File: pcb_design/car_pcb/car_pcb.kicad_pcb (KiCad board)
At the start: 2 copper layers, 158 x 115 mm, 28 parts, among them J1 PICO_R, J10 CMD_UART, J11 +5V, J12 PICO_L, J14 PWR_OUTPUT, J16 NRF24L01, J18 GND, J19 +3.3V, J2 PWR_INPUT, J20 GND, J21 PWR_IN_BTN, J22 Joystick_Y_PWR_GND, J23 Joystick_Y_SIGs, J24 Camera servo, J3 Joystick_X_PWR_GND, J4 Joystick_X_SIGs, J5 Motor_1, J6 Motor_2, J7 Motor_3, J8 Motor_4, J9 Debug_UART, U2 Mini360_5V, U3 Mini360_3.3V, U4 module_mpu6050, U5 ROB-14450

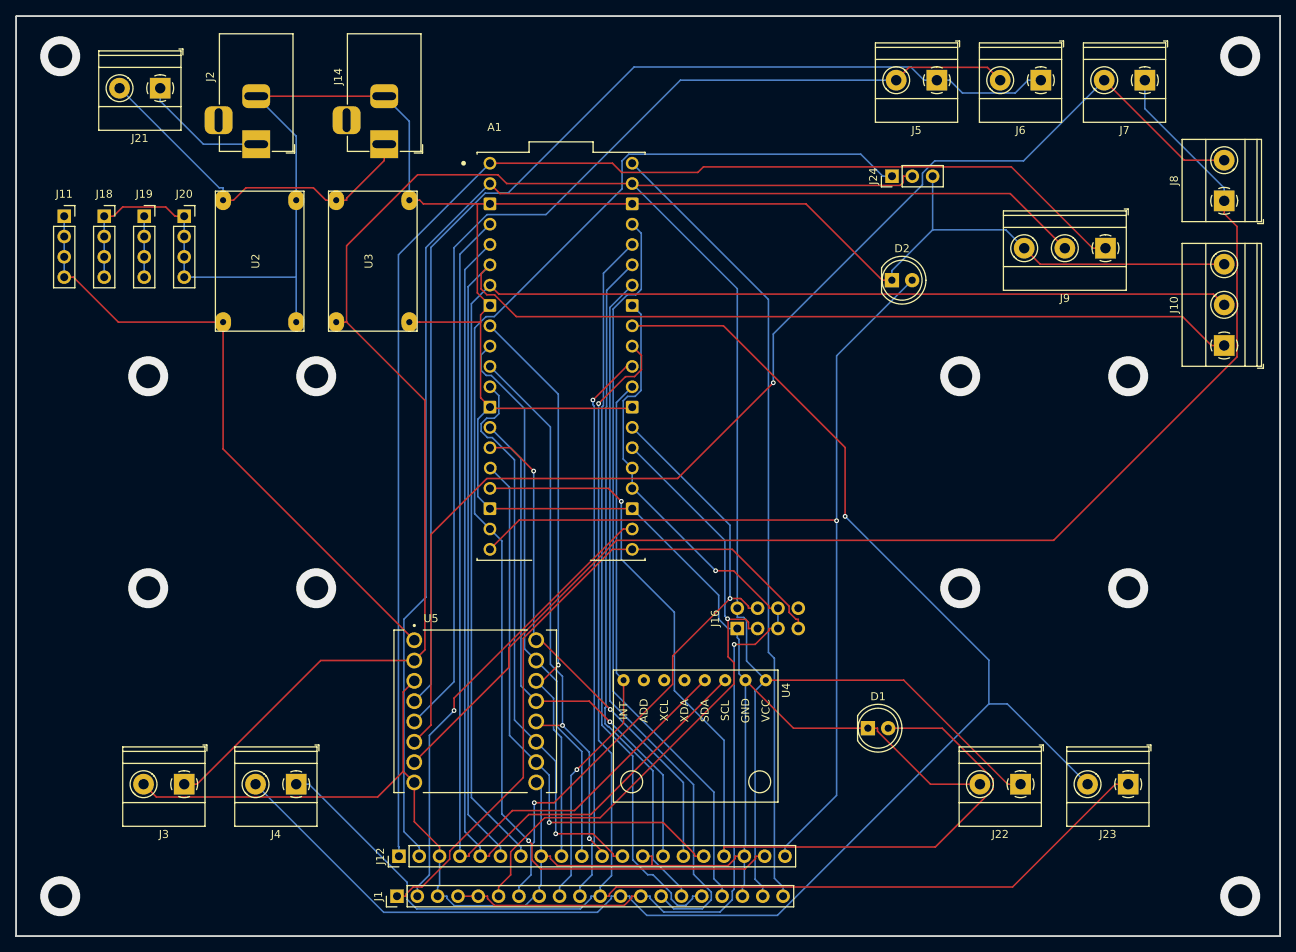
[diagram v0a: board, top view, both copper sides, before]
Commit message: update pcbs
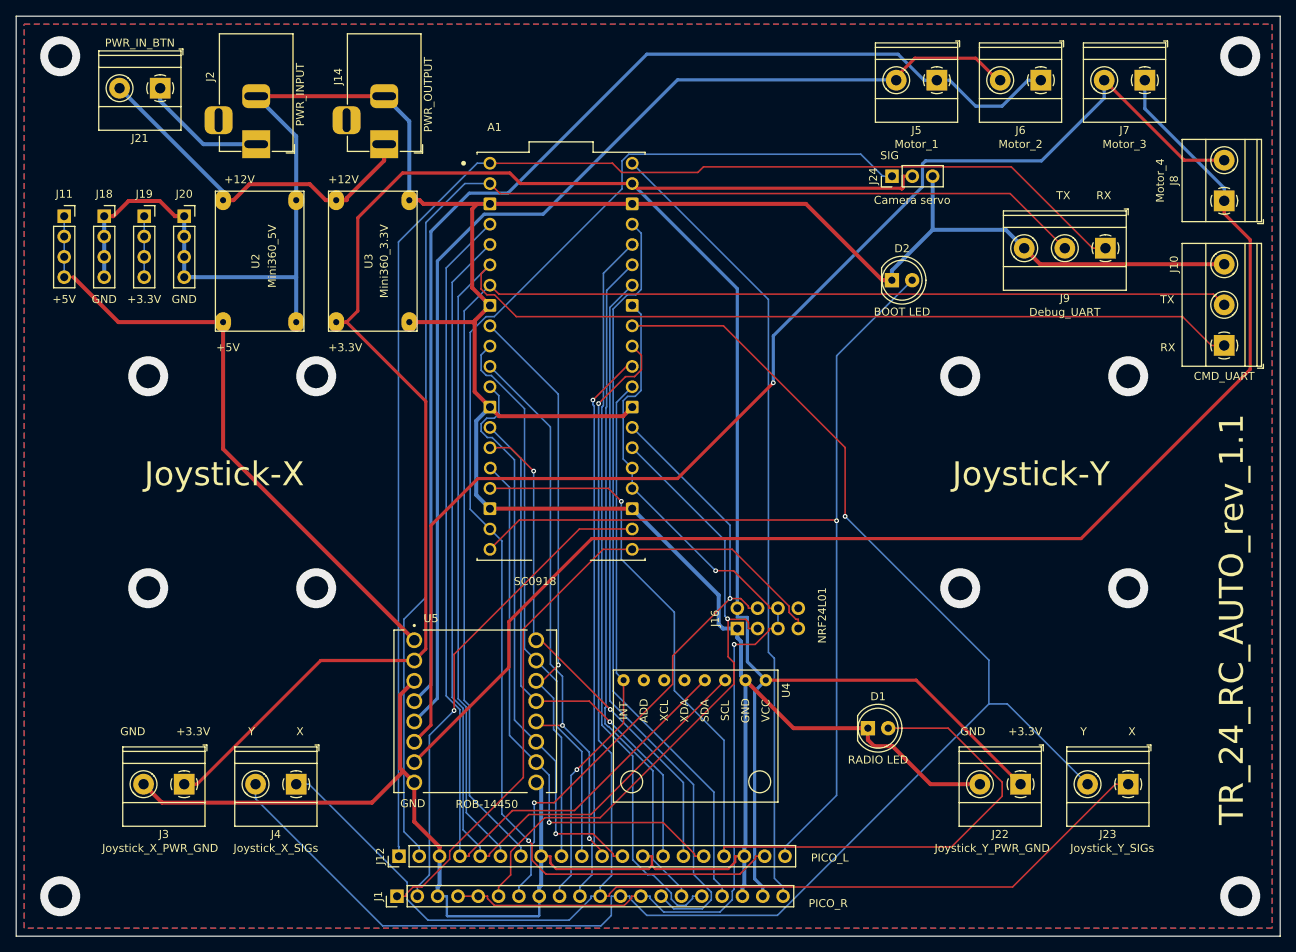
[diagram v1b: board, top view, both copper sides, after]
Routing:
- net GND: track 515.9 -> 525.2 mm
- net Net-(J7-Pin_1): track 164.6 -> 169.8 mm
- net Net-(J5-Pin_1): track 145.2 -> 149.0 mm
- net Net-(A1-GP27): track 200.3 -> 204.0 mm
- net Net-(A1-GP17): track 57.7 -> 60.9 mm
- net Net-(J7-Pin_2): track 158.0 -> 160.7 mm
- net +3.3V: track 303.4 -> 306.0 mm
- net Net-(A1-GP13): track 121.6 -> 124.1 mm
- net Net-(A1-GP1): track 164.5 -> 166.4 mm
- net Net-(A1-GP2): track 120.5 -> 121.9 mm
- net Net-(A1-GP3): track 118.5 -> 119.8 mm
- net Net-(A1-GP26): track 191.9 -> 193.0 mm
- net Net-(J5-Pin_2): track 139.6 -> 140.7 mm
- net Net-(A1-GP4): track 176.0 -> 177.0 mm
- net Net-(A1-GP14): track 164.2 -> 165.2 mm
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- added copper zone on B.Cu, net GND
- added copper zone on F.Cu, net GND
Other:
- board text added: "+12V"
- board text added: "+3.3V"
- board text added: "+5V"
- board text added: "GND"
- board text added: "Joystick-X"
- board text added: "Joystick-Y"
- board text added: "RX"
- board text added: "SIG"
- board text added: "TR_24_RC_AUTO_rev_1.1"
- board text added: "TX"
- board text added: "X"
- board text added: "Y"

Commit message: update pcbs
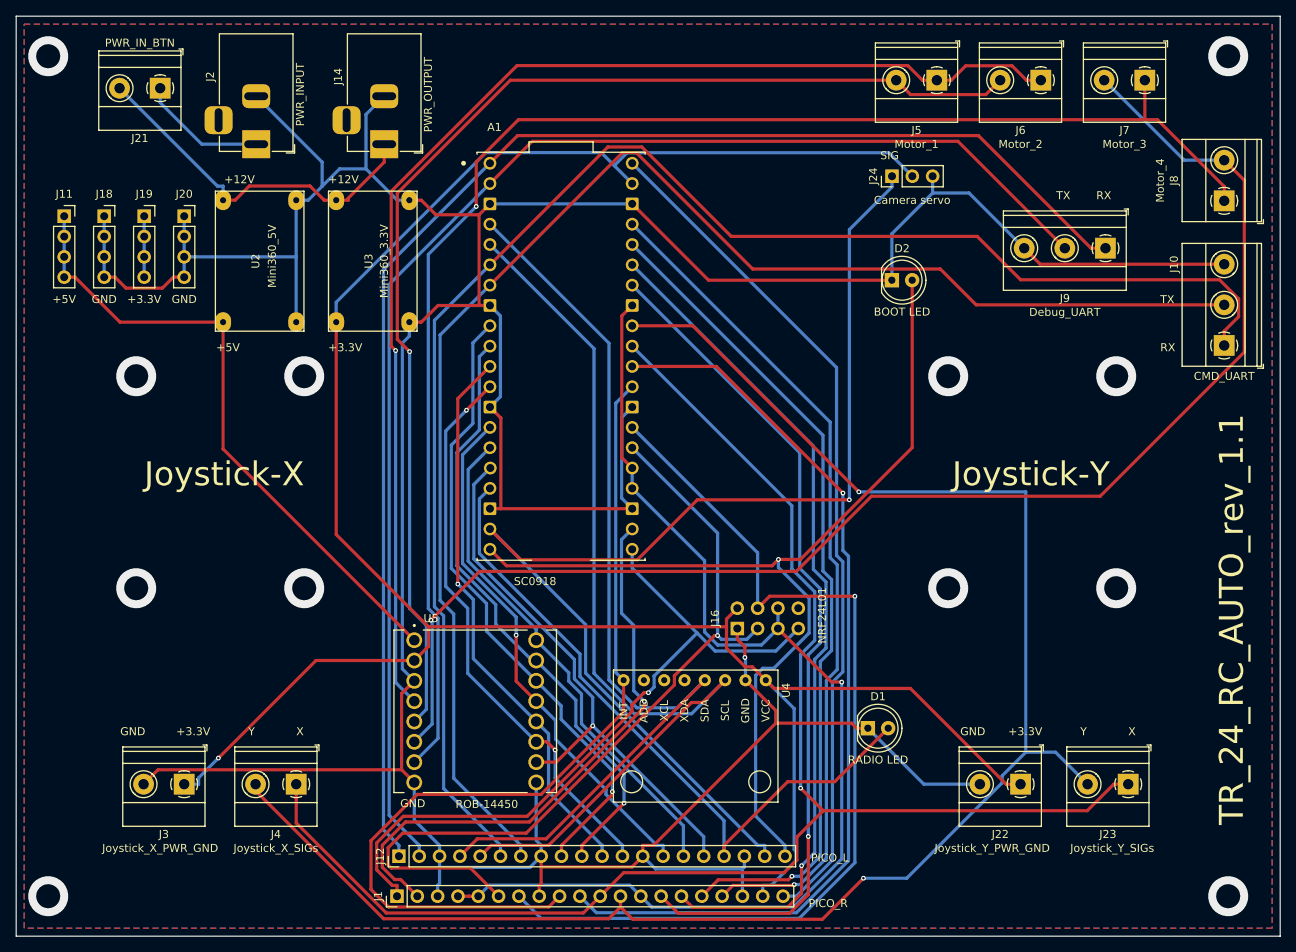
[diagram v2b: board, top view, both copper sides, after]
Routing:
- net Net-(A1-RUN): track 69.5 -> 116.3 mm
- net Net-(A1-GP22): track 68.2 -> 111.3 mm, vias 1 -> 0
- net Net-(A1-GP21): track 80.1 -> 121.2 mm, vias 2 -> 1
- net Net-(A1-GP13): track 124.1 -> 87.1 mm, vias 1 -> 0
- net Net-(A1-GP20): track 82.2 -> 104.1 mm
- net Net-(A1-ADC_VREF): track 84.4 -> 106.2 mm, vias 0 -> 1
- net Net-(A1-GP14): track 165.2 -> 147.9 mm
- net Net-(A1-GP4): track 177.0 -> 194.3 mm
- net +3.3V: track 306.0 -> 288.9 mm, vias 0 -> 1
- net Net-(A1-GP5): track 168.4 -> 184.7 mm
- net Net-(A1-GP28): track 90.6 -> 106.8 mm, vias 0 -> 1
- net Net-(A1-AGND): track 128.0 -> 143.9 mm, vias 2 -> 1
- net Net-(J7-Pin_1): track 169.8 -> 185.1 mm, vias 0 -> 1
- net Net-(J7-Pin_2): track 160.7 -> 175.9 mm
- net Net-(A1-3V3_EN): track 92.2 -> 105.4 mm, vias 0 -> 1
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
